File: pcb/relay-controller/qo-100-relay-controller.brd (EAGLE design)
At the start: 85 x 83.8 mm, 125 parts, among them CON1 4P-SH-SIDE, CON10 2EDG-2P-5MM, CON11 2EDG-2P-5MM, CON12 2EDG-2P-5MM, CON13 2EDG-2P-5MM, CON14 2EDG-2P-5MM, CON2 2EDG-2P-5MM, CON3 2EDG-2P-5MM, CON4 2EDG-2P-5MM, CON5 2EDG-2P-5MM, CON6 2EDG-2P-5MM, CON7 2EDG-2P-5MM, CON8 2EDG-2P-5MM, CON9 2EDG-2P-5MM, Q1 AO3400, Q10 AO3400, Q11 AO3400, Q12 AO3400, Q2 AO3400, Q3 AO3400, Q4 AO3400, Q5 AO3400, Q6 AO3400, Q7 AO3400, Q8 AO3400, Q9 AO3400, U1 MCP1792-3.3, U2 MCP23017

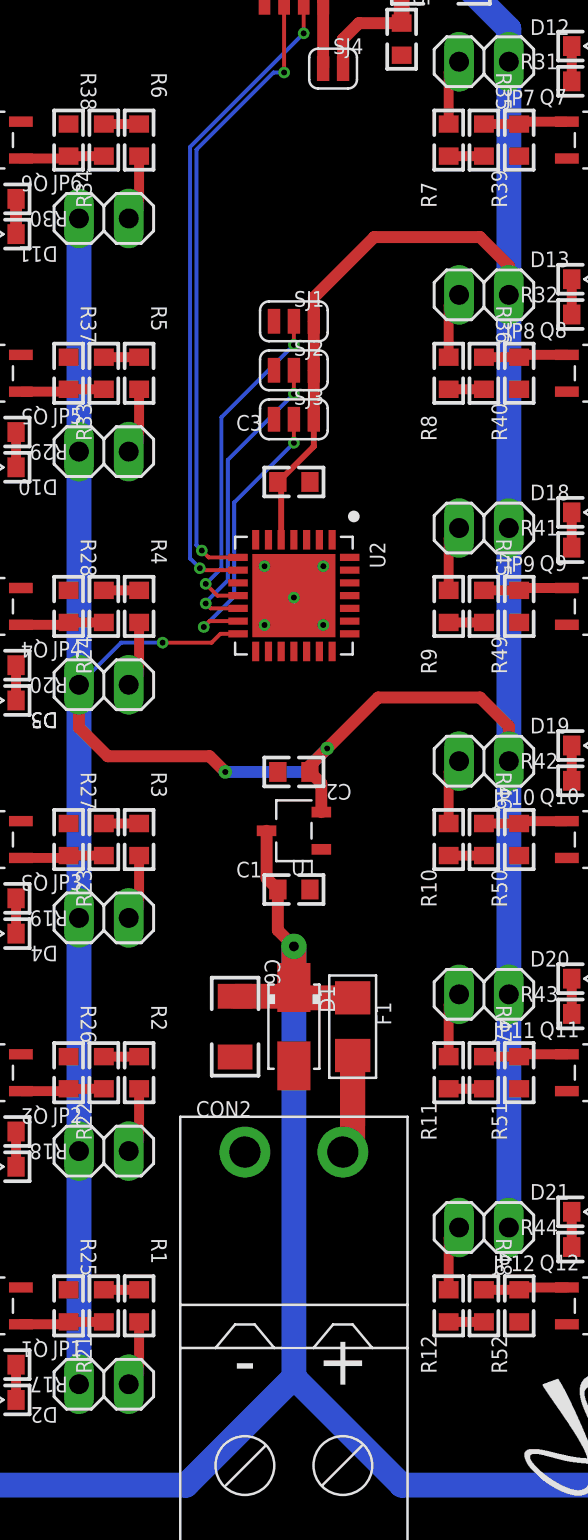
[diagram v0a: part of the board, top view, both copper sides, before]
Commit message: Nothing to do on Relay Controller
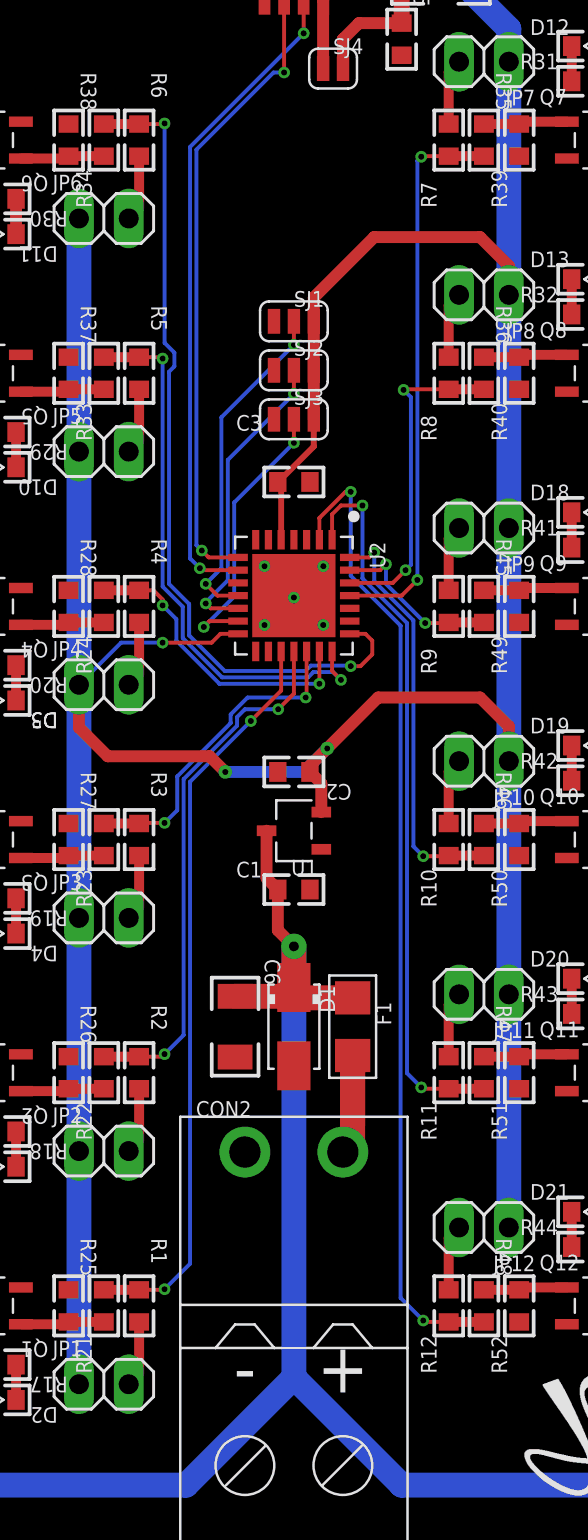
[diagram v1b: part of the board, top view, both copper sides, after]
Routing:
- net R11: track 1.80 -> 50.2 mm, vias 0 -> 2
- net R5: track 1.80 -> 42.5 mm, vias 0 -> 2
- net R0: track 1.80 -> 38.1 mm, vias 0 -> 2
- net R10: track 1.80 -> 37.2 mm, vias 0 -> 2
- net R6: track 1.80 -> 28.7 mm, vias 0 -> 2
- net R4: track 1.80 -> 28.5 mm, vias 0 -> 2
- net R1: track 1.80 -> 27.4 mm, vias 0 -> 2
- net R9: track 1.80 -> 21.0 mm, vias 0 -> 2
- net R7: track 1.80 -> 16.7 mm, vias 0 -> 2
- net R2: track 1.80 -> 16.6 mm, vias 0 -> 2
- net R3: track 1.80 -> 15.4 mm, vias 0 -> 2
- net R8: track 1.80 -> 8.82 mm, vias 0 -> 2
